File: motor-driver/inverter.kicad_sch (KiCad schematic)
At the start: 24 parts, among them Q10 NMOS, Q11 NMOS, Q12 NMOS, Q7 NMOS, Q8 NMOS, Q9 NMOS

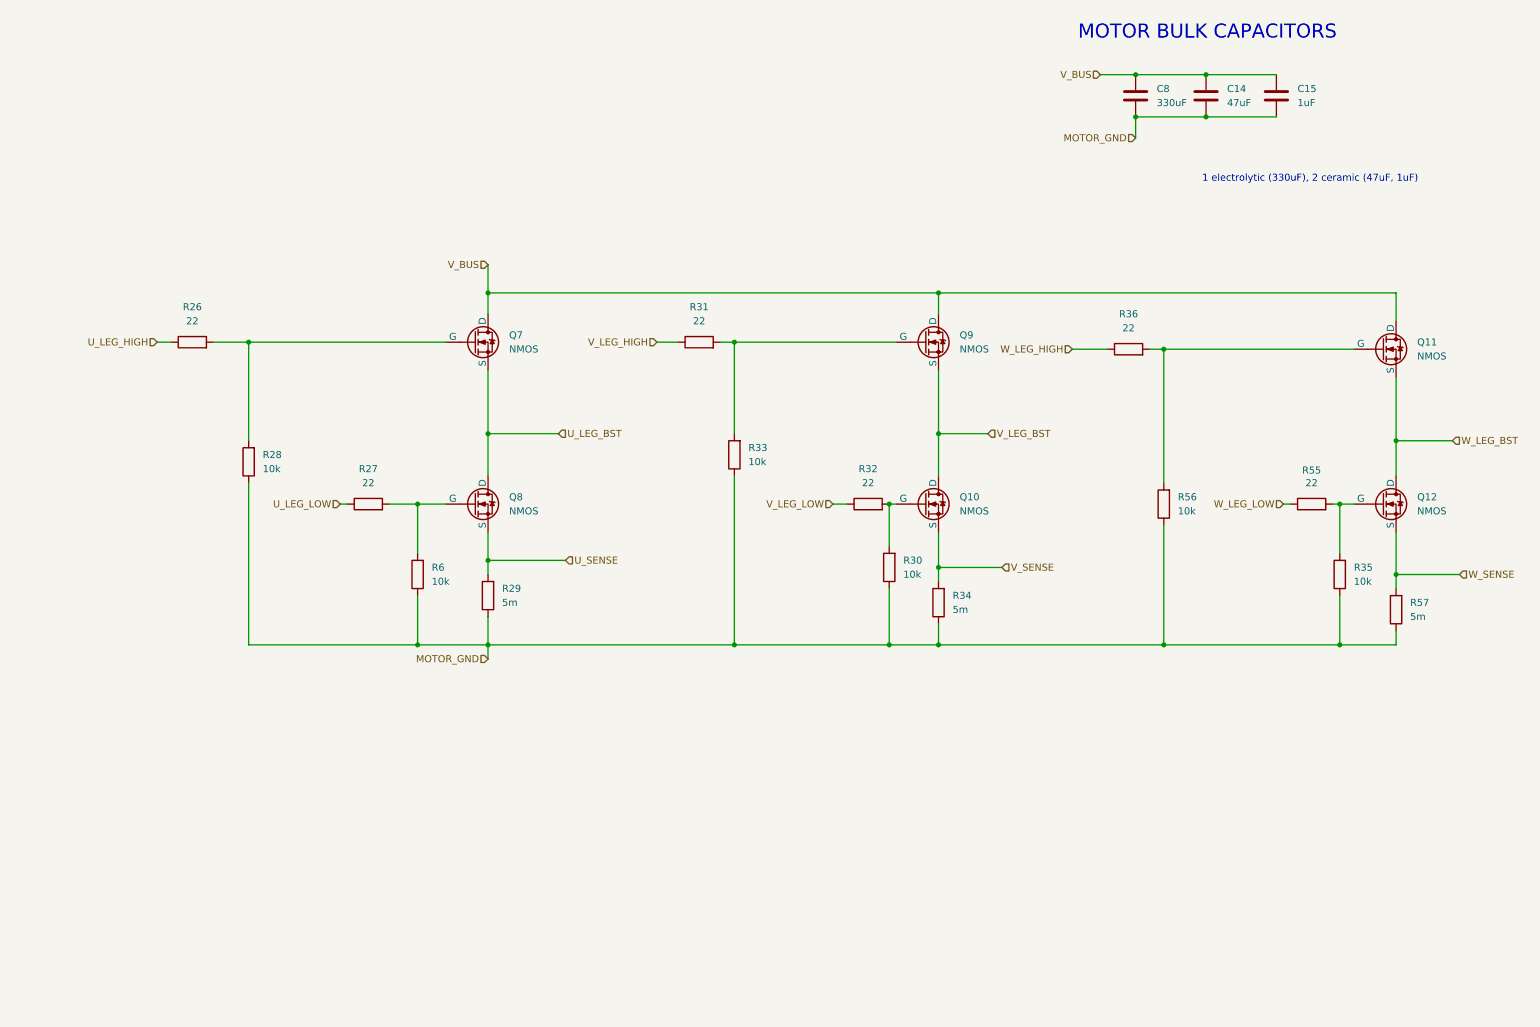
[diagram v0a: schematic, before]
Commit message: commit before changing custom sullen key sense
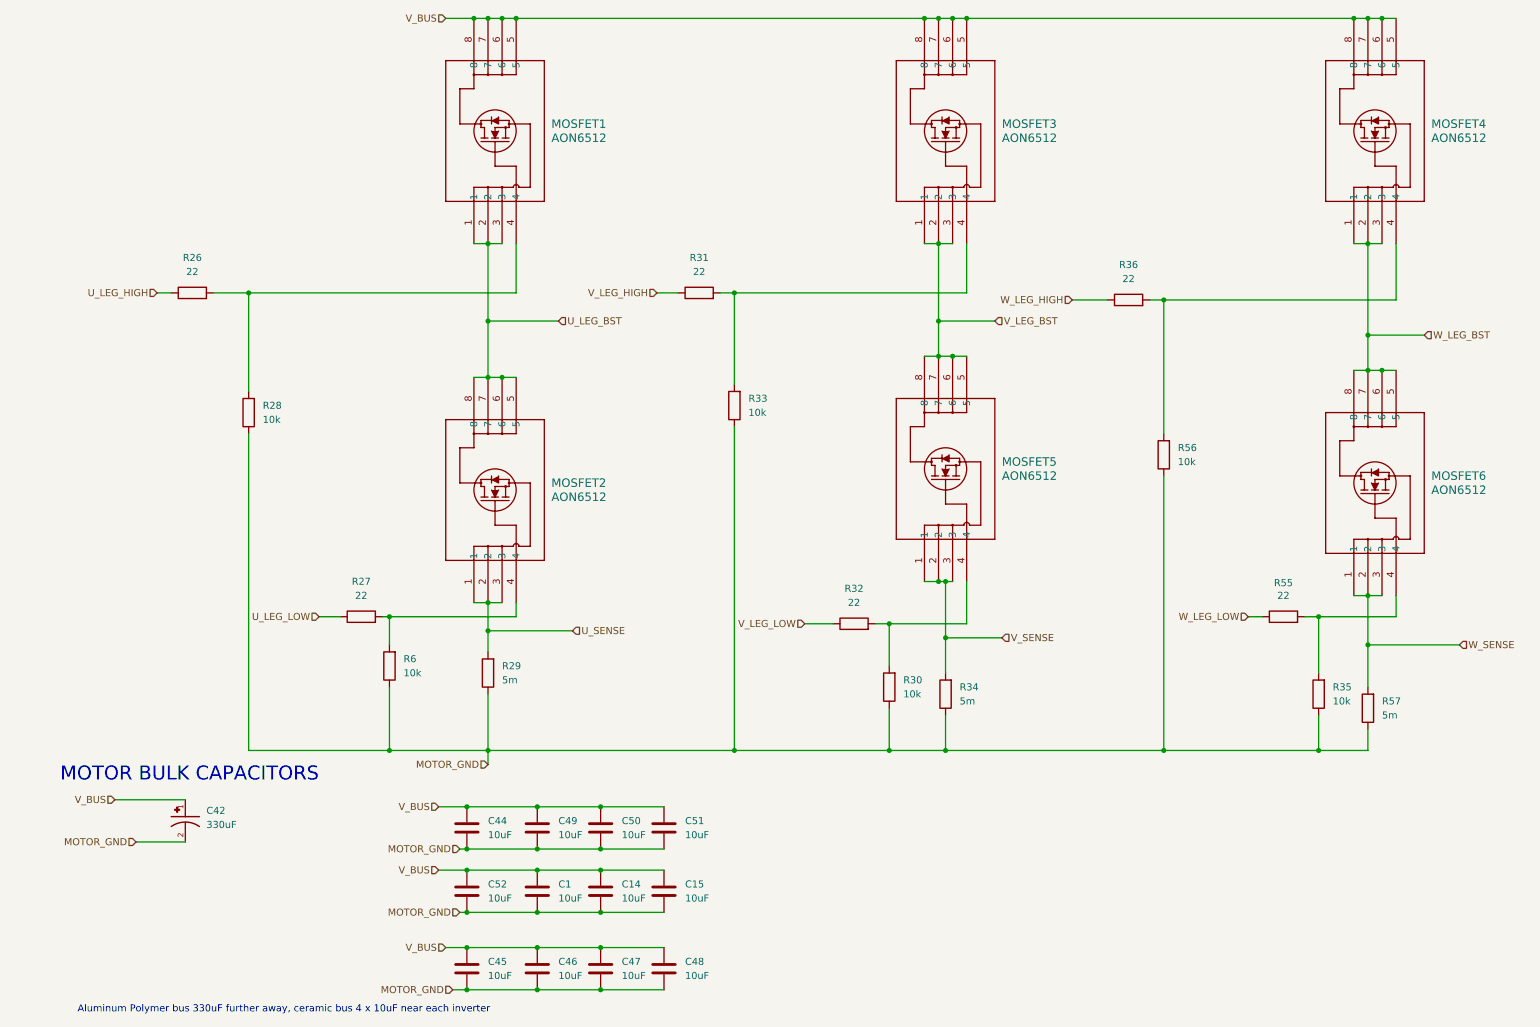
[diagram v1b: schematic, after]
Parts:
- removed C8: 330uF, 330uFCap:CAPPRD500W60D1000H1400, symbol Device:C
- removed Q10, Q11, Q12, Q7, Q8, Q9: NMOS, IPD090N03L:DPAK228P998X235-3N, symbol Simulation_SPICE:NMOS
- added C1, C44, C45, C46, C47, C48, C49, C50, C51, C52: 10uF, Capacitor_SMD:C_0603_1608Metric, symbol Device:C
- added C42: 330uF, A768MS337M1VLAS022:CAPAE1030X1225N, symbol A768MS337M1VLAS022:A768MS337M1VLAS022
- added MOSFET1, MOSFET2, MOSFET3, MOSFET4, MOSFET5, MOSFET6: AON6512, AON6512:DFN5X6_8L_EP1_P_AOS, symbol AON6512:AON6512
- C14: value 47uF -> 10uF; footprint Capacitor_SMD:C_0201_0603Metric_Pad0.64x0.40mm_HandSolder -> Capacitor_SMD:C_0603_1608Metric
- C15: value 1uF -> 10uF; footprint Capacitor_SMD:C_0201_0603Metric_Pad0.64x0.40mm_HandSolder -> Capacitor_SMD:C_0603_1608Metric
- R26, R27, R28, R30, R31, R32, R33, R35, R36, R55, R56, R6: footprint Resistor_SMD:R_0805_2012Metric -> Resistor_SMD:R_0603_1608Metric
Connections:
- net MOTOR_GND: now also C1.2, C42.2, C44.2, C45.2, C46.2, C47.2, C48.2, C49.2, C50.2, C51.2, C52.2
- net U_LEG_BST: now also MOSFET1.1, MOSFET1.2, MOSFET1.3, MOSFET2.5, MOSFET2.6, MOSFET2.7, MOSFET2.8
- net U_SENSE: now also MOSFET2.1, MOSFET2.2, MOSFET2.3
- net V_BUS: now also C1.1, C42.1, C44.1, C45.1, C46.1, C47.1, C48.1, C49.1, C50.1, C51.1, C52.1, MOSFET1.5, MOSFET1.6, MOSFET1.7, MOSFET1.8, MOSFET3.5, MOSFET3.6, MOSFET3.7, MOSFET3.8, MOSFET4.5, MOSFET4.6, MOSFET4.7, MOSFET4.8
- net V_LEG_BST: now also MOSFET3.1, MOSFET3.2, MOSFET3.3, MOSFET5.5, MOSFET5.6, MOSFET5.7, MOSFET5.8
- net V_SENSE: now also MOSFET5.1, MOSFET5.2, MOSFET5.3
- net W_LEG_BST: now also MOSFET4.1, MOSFET4.2, MOSFET4.3, MOSFET6.5, MOSFET6.6, MOSFET6.7, MOSFET6.8
- net W_SENSE: now also MOSFET6.1, MOSFET6.2, MOSFET6.3
- net at R26.2, R28.2: now also MOSFET1.4
- net at R36.2, R56.2: now also MOSFET4.4
- net at R35.2, R55.2: now also MOSFET6.4
- net at R27.2, R6.2: now also MOSFET2.4
- net at R31.2, R33.2: now also MOSFET3.4
- net at R30.2, R32.2: now also MOSFET5.4
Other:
- note added: "Aluminum Polymer bus 330uF further away, ceramic bus 4 x 10uF near each inverter"
- note removed: "1 electrolytic (330uF), 2 ceramic (47uF, 1uF)"
- moved on the sheet: R26, R27, R28, R29, R30, R31, R32, R33, R34, R35, R36, R55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
